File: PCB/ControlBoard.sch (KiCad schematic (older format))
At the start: 15 parts, among them J1 Conn_01x02, J2 Conn_01x12, SW1 SW_Push, SW2 SW_Push, SW3 SW_Push, U1 Nokia_5510_display_module

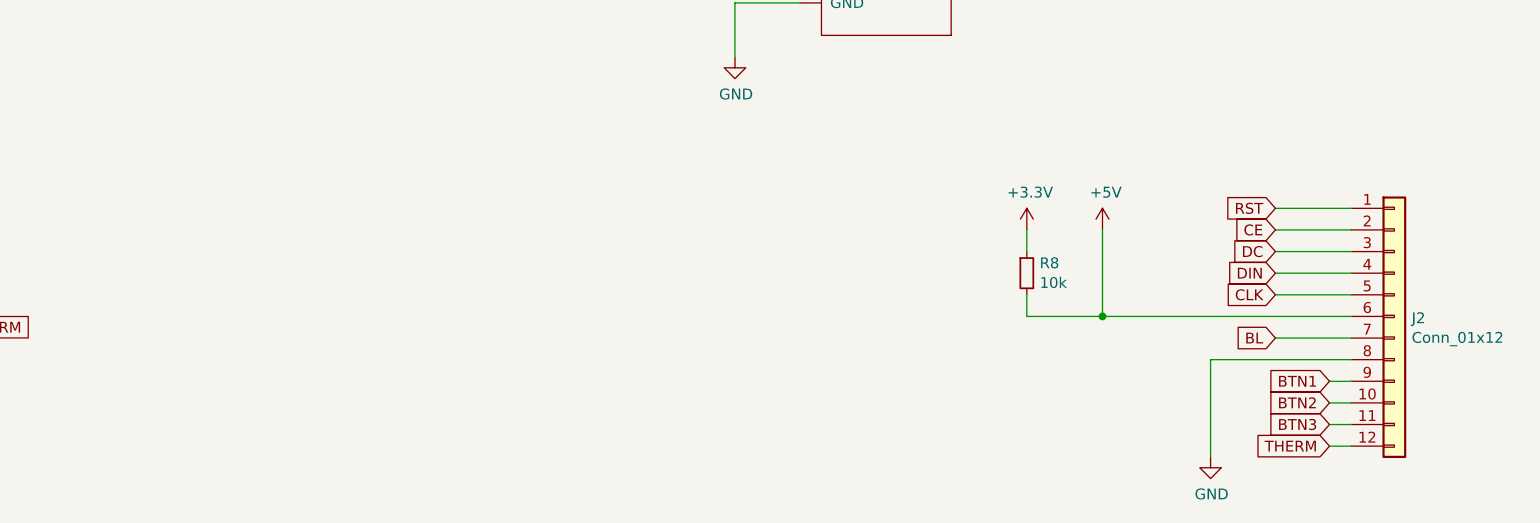
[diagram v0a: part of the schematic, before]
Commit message: Board done
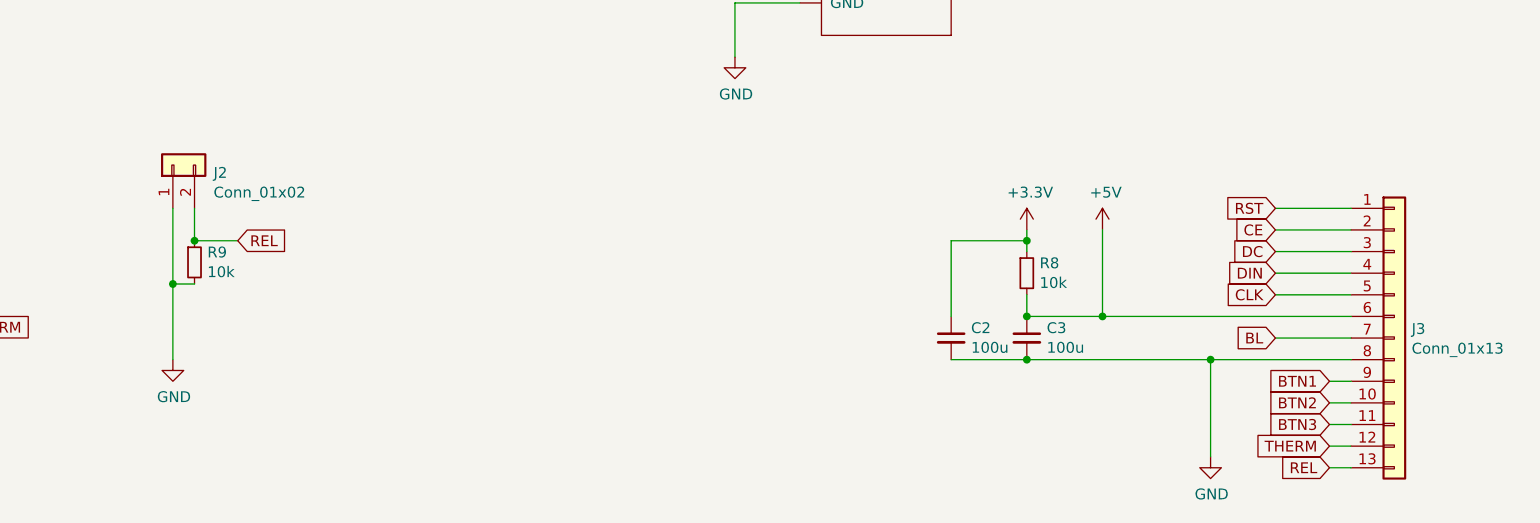
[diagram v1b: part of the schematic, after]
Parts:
- removed J2: Conn_01x12, Connector_PinHeader_2.54mm:PinHeader_1x12_P2.54mm_Vertical, symbol Connector_Generic:Conn_01x12
- added C2, C3: 100u, Capacitor_SMD:C_0603_1608Metric_Pad1.08x0.95mm_HandSolder, symbol Device:C_Small
- added J2: Conn_01x02, Connector_PinHeader_2.54mm:PinHeader_1x02_P2.54mm_Horizontal, symbol Connector_Generic:Conn_01x02
- added J3: Conn_01x13, Connector_PinHeader_2.54mm:PinHeader_1x13_P2.54mm_Vertical, symbol Connector_Generic:Conn_01x13
- added R9: 10k, Resistor_SMD:R_0402_1005Metric_Pad0.72x0.64mm_HandSolder, symbol Device:R_Small
- C1: footprint Capacitor_SMD:C_0201_0603Metric_Pad0.64x0.40mm_HandSolder -> Capacitor_SMD:C_0603_1608Metric_Pad1.08x0.95mm_HandSolder
- R1, R2, R3, R4, R5, R6, R7, R8: footprint Resistor_SMD:R_01005_0402Metric_Pad0.57x0.30mm_HandSolder -> Resistor_SMD:R_0402_1005Metric_Pad0.72x0.64mm_HandSolder
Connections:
- net +3V3: now also C2.1
- net +5V: now also C3.1, J3.6 (Pin_6)
- net BL: now also J3.7 (Pin_7)
- net BTN1: now also J3.9 (Pin_9)
- net BTN2: now also J3.10 (Pin_10)
- net BTN3: now also J3.11 (Pin_11)
- net CE: now also J3.2 (Pin_2)
- net CLK: now also J3.5 (Pin_5)
- net DC: now also J3.3 (Pin_3)
- net DIN: now also J3.4 (Pin_4)
- net GND: now also C2.2, C3.2, J2.1 (Pin_1), J3.8 (Pin_8), R9.2
- net RST: now also J3.1 (Pin_1)
- net THERM: now also J3.12 (Pin_12)
- new net REL: J2.2 (Pin_2), J3.13 (Pin_13), R9.1
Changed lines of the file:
@@
 F 0 "R4" H 6409 3596 50  0000 L CNN
 F 1 "10k" H 6409 3505 50  0000 L CNN
-F 2 "Resistor_SMD:R_01005_0402Metric_Pad0.57x0.30mm_HandSolder" H 6350 3550 50  0001 C CNN
+F 2 "Resistor_SMD:R_0402_1005Metric_Pad0.72x0.64mm_HandSolder" H 6350 3550 50  0001 C CNN
 F 3 "~" H 6350 3550 50  0001 C CNN
 	1    6350 3550
@@
 F 0 "R3" V 6296 3650 50  0000 C CNN
 F 1 "10k" V 6205 3650 50  0000 C CNN
-F 2 "Resistor_SMD:R_01005_0402Metric_Pad0.57x0.30mm_HandSolder" H 6100 3650 50  0001 C CNN
+F 2 "Resistor_SMD:R_0402_1005Metric_Pad0.72x0.64mm_HandSolder" H 6100 3650 50  0001 C CNN
 F 3 "~" H 6100 3650 50  0001 C CNN
 	1    6100 3650
@@
 F 0 "R2" V 6046 3750 50  0000 C CNN
 F 1 "10k" V 5955 3750 50  0000 C CNN
-F 2 "Resistor_SMD:R_01005_0402Metric_Pad0.57x0.30mm_HandSolder" H 5850 3750 50  0001 C CNN
+F 2 "Resistor_SMD:R_0402_1005Metric_Pad0.72x0.64mm_HandSolder" H 5850 3750 50  0001 C CNN
 F 3 "~" H 5850 3750 50  0001 C CNN
 	1    5850 3750
@@
 F 0 "R6" V 6846 3950 50  0000 C CNN
 F 1 "440" V 6755 3950 50  0000 C CNN
-F 2 "Resistor_SMD:R_01005_0402Metric_Pad0.57x0.30mm_HandSolder" H 6650 3950 50  0001 C CNN
+F 2 "Resistor_SMD:R_0402_1005Metric_Pad0.72x0.64mm_HandSolder" H 6650 3950 50  0001 C CNN
 F 3 "~" H 6650 3950 50  0001 C CNN
 	1    6650 3950
@@
 F 0 "R7" V 7146 3350 50  0000 C CNN
 F 1 "10k" V 7055 3350 50  0000 C CNN
-F 2 "Resistor_SMD:R_01005_0402Metric_Pad0.57x0.30mm_HandSolder" H 6950 3350 50  0001 C CNN
+F 2 "Resistor_SMD:R_0402_1005Metric_Pad0.72x0.64mm_HandSolder" H 6950 3350 50  0001 C CNN
 F 3 "~" H 6950 3350 50  0001 C CNN
 	1    6950 3350
@@
 F 0 "R5" V 6454 3450 50  0000 C CNN
 F 1 "1k" V 6545 3450 50  0000 C CNN
-F 2 "Resistor_SMD:R_01005_0402Metric_Pad0.57x0.30mm_HandSolder" H 6650 3450 50  0001 C CNN
+F 2 "Resistor_SMD:R_0402_1005Metric_Pad0.72x0.64mm_HandSolder" H 6650 3450 50  0001 C CNN
 F 3 "~" H 6650 3450 50  0001 C CNN
 	1    6650 3450
@@
 	9800 5600 9450 5600
 $Comp
-L Connector_Generic:Conn_01x12 J2
-U 1 1 624724E7
-P 10000 5500
-F 0 "J2" H 10080 5492 50  0000 L CNN
-F 1 "Conn_01x12" H 10080 5401 50  0000 L CNN
-F 2 "Connector_PinHeader_2.54mm:PinHeader_1x12_P2.54mm_Vertical" H 10000 5500 50  0001 C CNN
-F 3 "~" H 10000 5500 50  0001 C CNN
-	1    10000 5500
-	1    0    0    -1
-$EndComp
-$Comp
 L power:GND #PWR0103
 U 1 1 62475100
@@
 	1    0    0    -1
 $EndComp
-Wire Wire Line
-	9150 6150 9150 5700
 Wire Wire Line
 	9150 5700 9800 5700
@@
 F 0 "R1" H 2809 5496 50  0000 L CNN
 F 1 "4.7k" H 2809 5405 50  0000 L CNN
-F 2 "Resistor_SMD:R_01005_0402Metric_Pad0.57x0.30mm_HandSolder" H 2750 5450 50  0001 C CNN
+F 2 "Resistor_SMD:R_0402_1005Metric_Pad0.72x0.64mm_HandSolder" H 2750 5450 50  0001 C CNN
 F 3 "~" H 2750 5450 50  0001 C CNN
 	1    2750 5450
@@
 F 0 "C1" H 2842 5746 50  0000 L CNN
 F 1 "10uF" H 2842 5655 50  0000 L CNN
-F 2 "Capacitor_SMD:C_0201_0603Metric_Pad0.64x0.40mm_HandSolder" H 2750 5700 50  0001 C CNN
+F 2 "Capacitor_SMD:C_0603_1608Metric_Pad1.08x0.95mm_HandSolder" H 2750 5700 50  0001 C CNN
 F 3 "~" H 2750 5700 50  0001 C CNN
 	1    2750 5700
@@
 F 0 "R8" H 8359 5346 50  0000 L CNN
 F 1 "10k" H 8359 5255 50  0000 L CNN
-F 2 "Resistor_SMD:R_01005_0402Metric_Pad0.57x0.30mm_HandSolder" H 8300 5300 50  0001 C CNN
+F 2 "Resistor_SMD:R_0402_1005Metric_Pad0.72x0.64mm_HandSolder" H 8300 5300 50  0001 C CNN
 F 3 "~" H 8300 5300 50  0001 C CNN
 	1    8300 5300
@@
 Connection ~ 8650 5500
 Wire Wire Line
-	8300 5200 8300 5100
+	8300 5200 8300 5150
+$Comp
+L Device:C_Small C3
+U 1 1 62474919
+P 8300 5600
+F 0 "C3" H 8392 5646 50  0000 L CNN
+F 1 "100u" H 8392 5555 50  0000 L CNN
+F 2 "Capacitor_SMD:C_0603_1608Metric_Pad1.08x0.95mm_HandSolder" H 8300 5600 50  0001 C CNN
+F 3 "~" H 8300 5600 50  0001 C CNN
+	1    8300 5600
+	1    0    0    -1
+$EndComp
+Connection ~ 8300 5500
+$Comp
+L Device:C_Small C2
+U 1 1 62475604
+P 7950 5600
+F 0 "C2" H 8042 5646 50  0000 L CNN
+F 1 "100u" H 8042 5555 50  0000 L CNN
+F 2 "Capacitor_SMD:C_0603_1608Metric_Pad1.08x0.95mm_HandSolder" H 7950 5600 50  0001 C CNN
+F 3 "~" H 7950 5600 50  0001 C CNN
+	1    7950 5600
+	1    0    0    -1
+$EndComp
+Wire Wire Line
+	8300 5700 9150 5700
+Connection ~ 9150 5700
+Wire Wire Line
+	8300 5700 7950 5700
+Connection ~ 8300 5700
+Wire Wire Line
+	7950 5500 7950 5150
+Wire Wire Line
+	7950 5150 8300 5150
+Wire Wire Line
+	9150 5700 9150 6150
+Connection ~ 8300 5150
+Wire Wire Line
+	8300 5150 8300 5100
+$Comp
+L Connector_Generic:Conn_01x13 J3
+U 1 1 6247934C
+P 10000 5600
+F 0 "J3" H 10080 5642 50  0000 L CNN
+F 1 "Conn_01x13" H 10080 5551 50  0000 L CNN
+F 2 "Connector_PinHeader_2.54mm:PinHeader_1x13_P2.54mm_Vertical" H 10000 5600 50  0001 C CNN
+F 3 "~" H 10000 5600 50  0001 C CNN
+	1    10000 5600
+	1    0    0    -1
+$EndComp
+Text GLabel 9700 6200 0    50   Input ~ 0
+REL
+Wire Wire Line
+	9800 6200 9700 6200
+$Comp
+L Connector_Generic:Conn_01x02 J2
+U 1 1 6247BBE1
+P 4350 4800
+F 0 "J2" V 4314 4612 50  0000 R CNN
+F 1 "Conn_01x02" V 4223 4612 50  0000 R CNN
+F 2 "Connector_PinHeader_2.54mm:PinHeader_1x02_P2.54mm_Horizontal" H 4350 4800 50  0001 C CNN
+F 3 "~" H 4350 4800 50  0001 C CNN
+	1    4350 4800
+	0    -1   -1   0
+$EndComp
+$Comp
+L power:GND #PWR0111
+U 1 1 6247C77E
+P 4350 5700
+F 0 "#PWR0111" H 4350 5450 50  0001 C CNN
+F 1 "GND" H 4355 5527 50  0000 C CNN
+F 2 "" H 4350 5700 50  0001 C CNN
+F 3 "" H 4350 5700 50  0001 C CNN
+	1    4350 5700
+	1    0    0    -1
+$EndComp
+Wire Wire Line
+	4350 5000 4350 5350
+Text GLabel 4650 5150 2    50   Input ~ 0
+REL
+Wire Wire Line
+	4450 5000 4450 5150
+Wire Wire Line
+	4450 5150 4650 5150
+$Comp
+L Device:R_Small R9
+U 1 1 624AA49D
+P 4450 5250
+F 0 "R9" H 4509 5296 50  0000 L CNN
+F 1 "10k" H 4509 5205 50  0000 L CNN
+F 2 "Resistor_SMD:R_0402_1005Metric_Pad0.72x0.64mm_HandSolder" H 4450 5250 50  0001 C CNN
+F 3 "~" H 4450 5250 50  0001 C CNN
+	1    4450 5250
+	1    0    0    -1
+$EndComp
+Connection ~ 4450 5150
+Wire Wire Line
+	4450 5350 4350 5350
+Connection ~ 4350 5350
+Wire Wire Line
+	4350 5350 4350 5700
 $EndSCHEMATC
